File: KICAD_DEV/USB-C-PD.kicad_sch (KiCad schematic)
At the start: 36 parts, among them J1 USB_C_Receptacle_USB2.0_14P, Q1 NMOS, U2 TPS26750, U3 TPD4S480

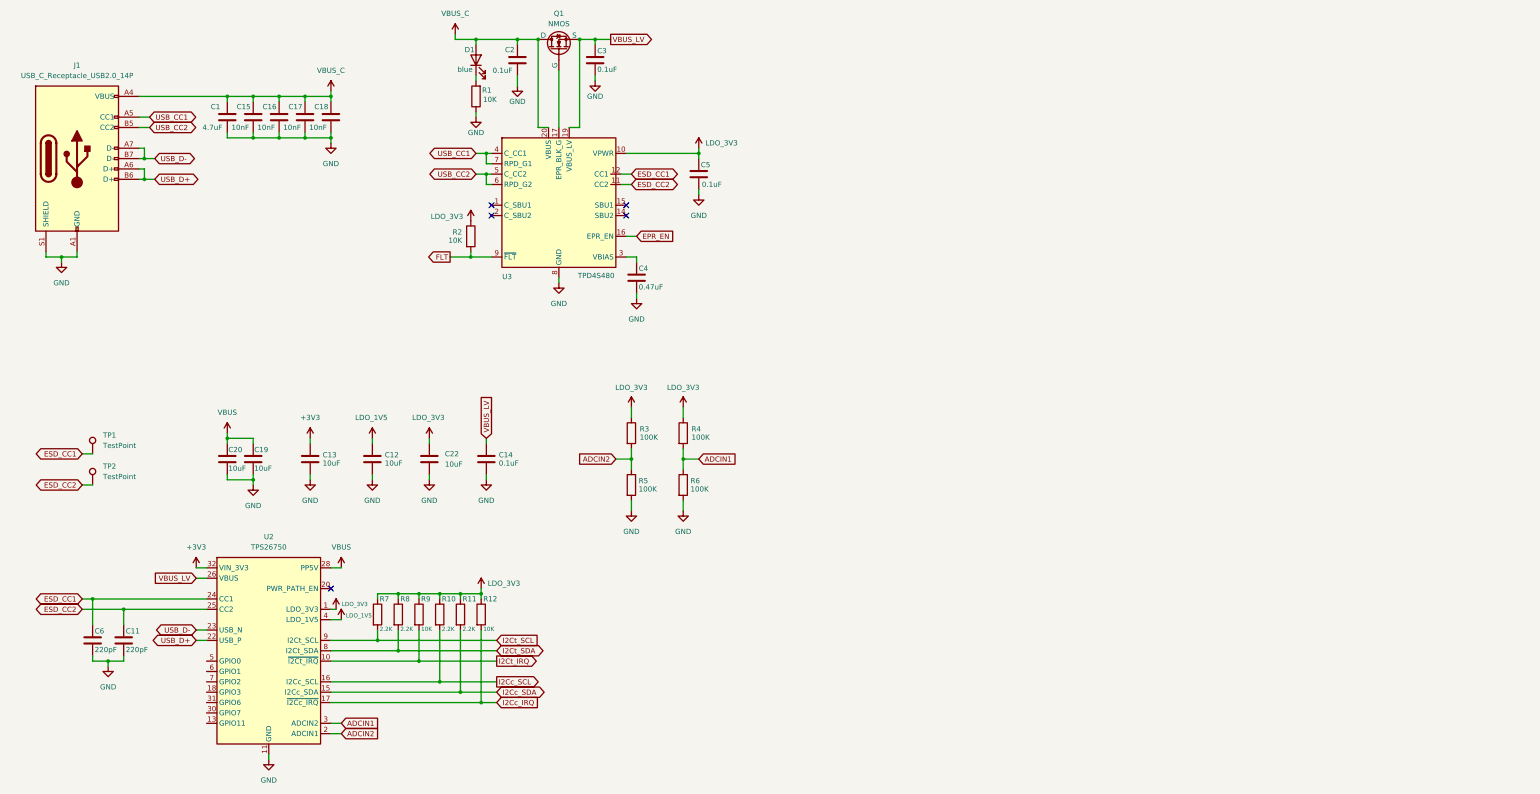
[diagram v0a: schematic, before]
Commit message: cooking
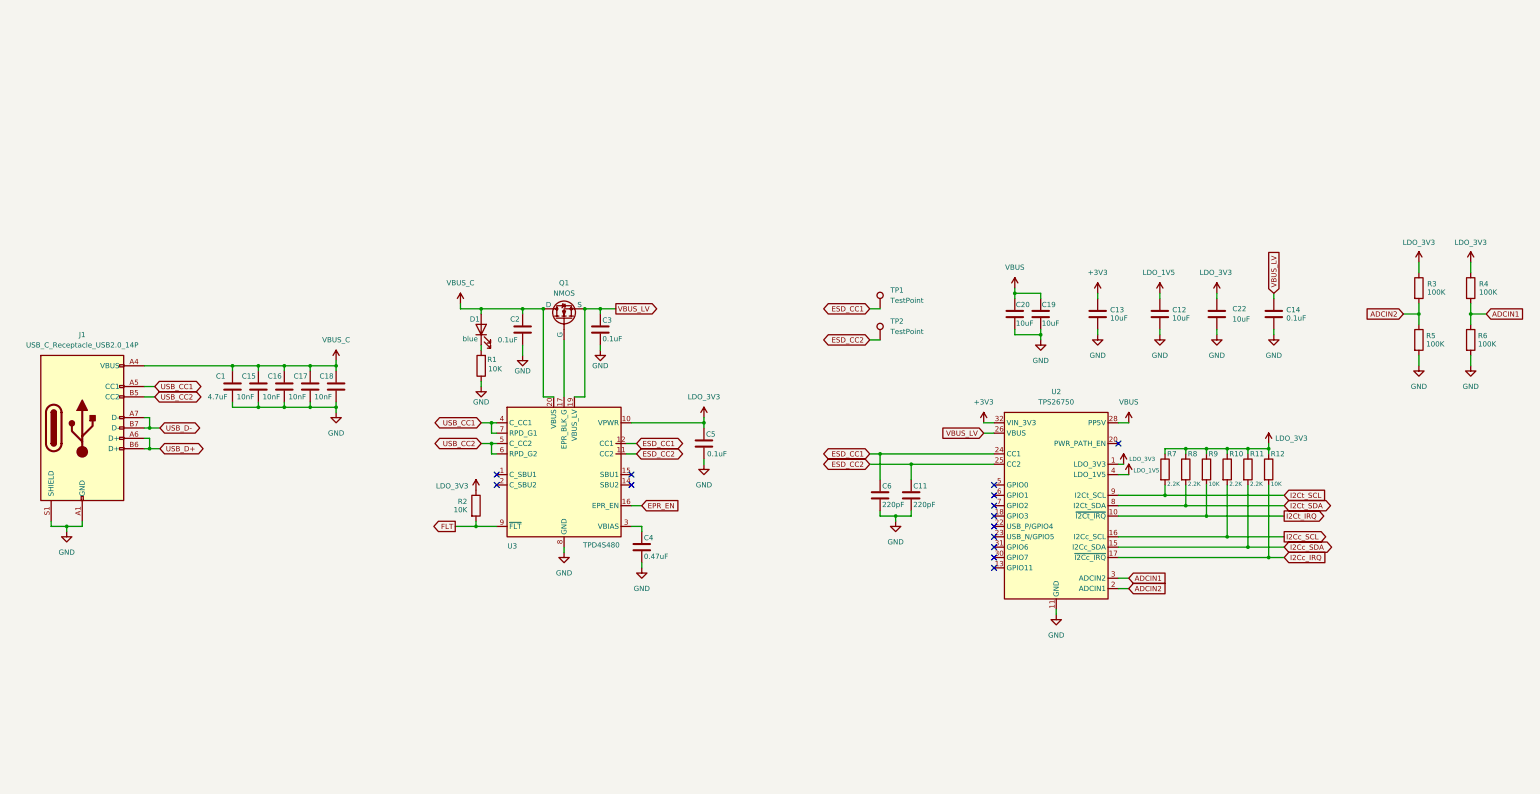
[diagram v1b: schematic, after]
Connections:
- net USB_D+: no longer U2.22 (USB_P)
- net USB_D-: no longer U2.23 (USB_N)
- no-connect marks 5 -> 14
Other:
- moved on the sheet: C1, C11, C12, C13, C14, C15, C16, C17, C18, C19, C2, C20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
